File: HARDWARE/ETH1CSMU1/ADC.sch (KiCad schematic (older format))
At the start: 25 parts, among them U1201 AD746, U1202 LTC6655-5, U1203 LTC2512-24, U1204 OP07, U1205 ADG5204_TSSOP

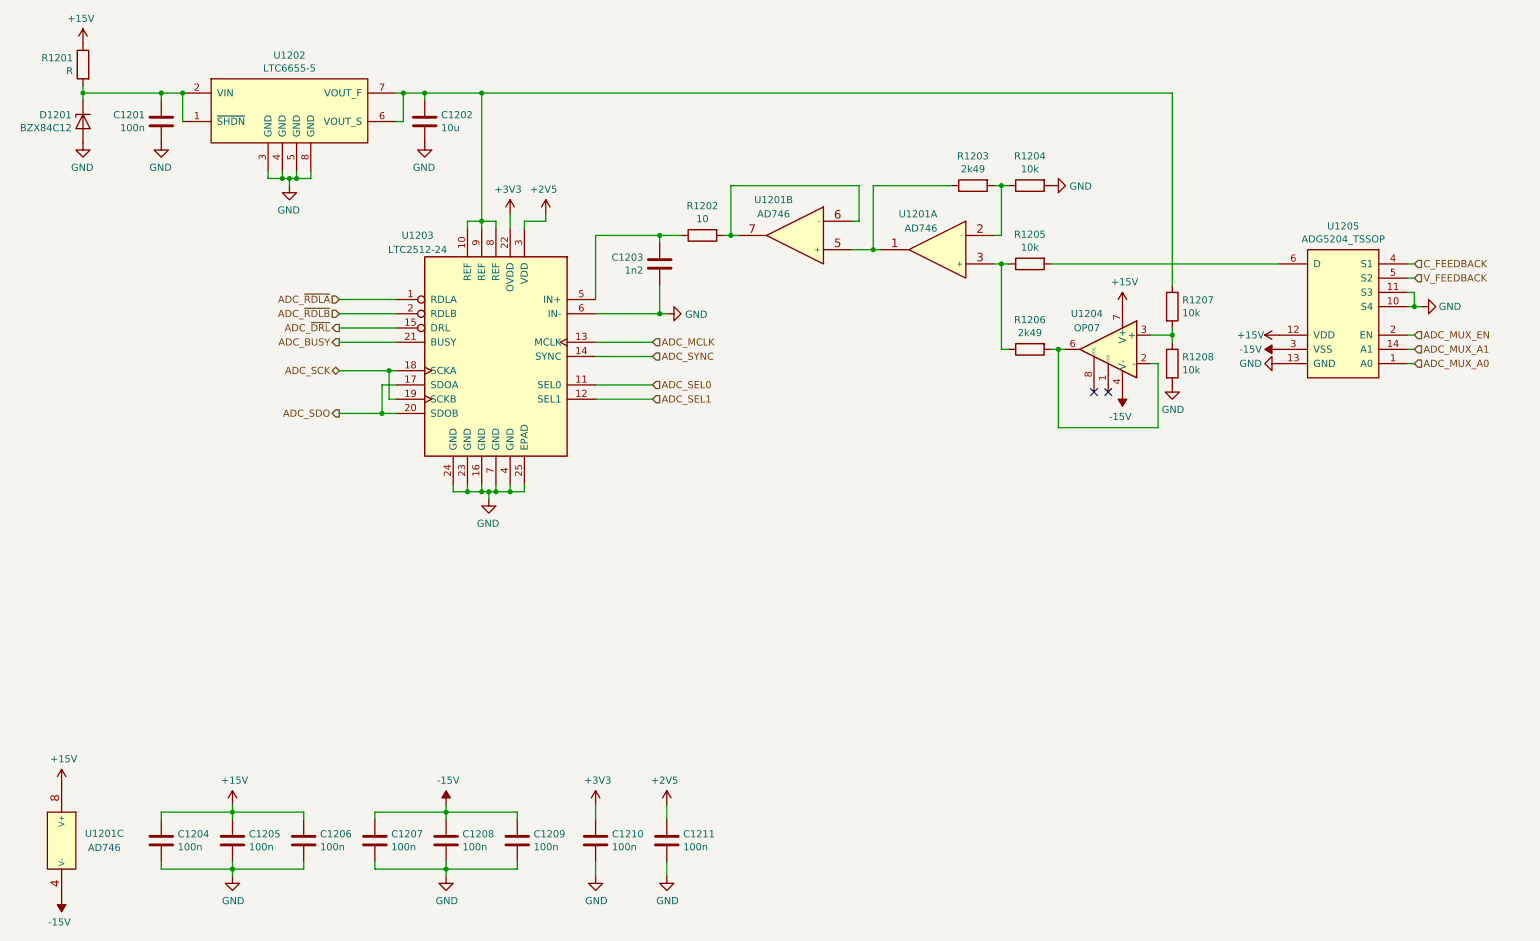
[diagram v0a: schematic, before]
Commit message: Commit
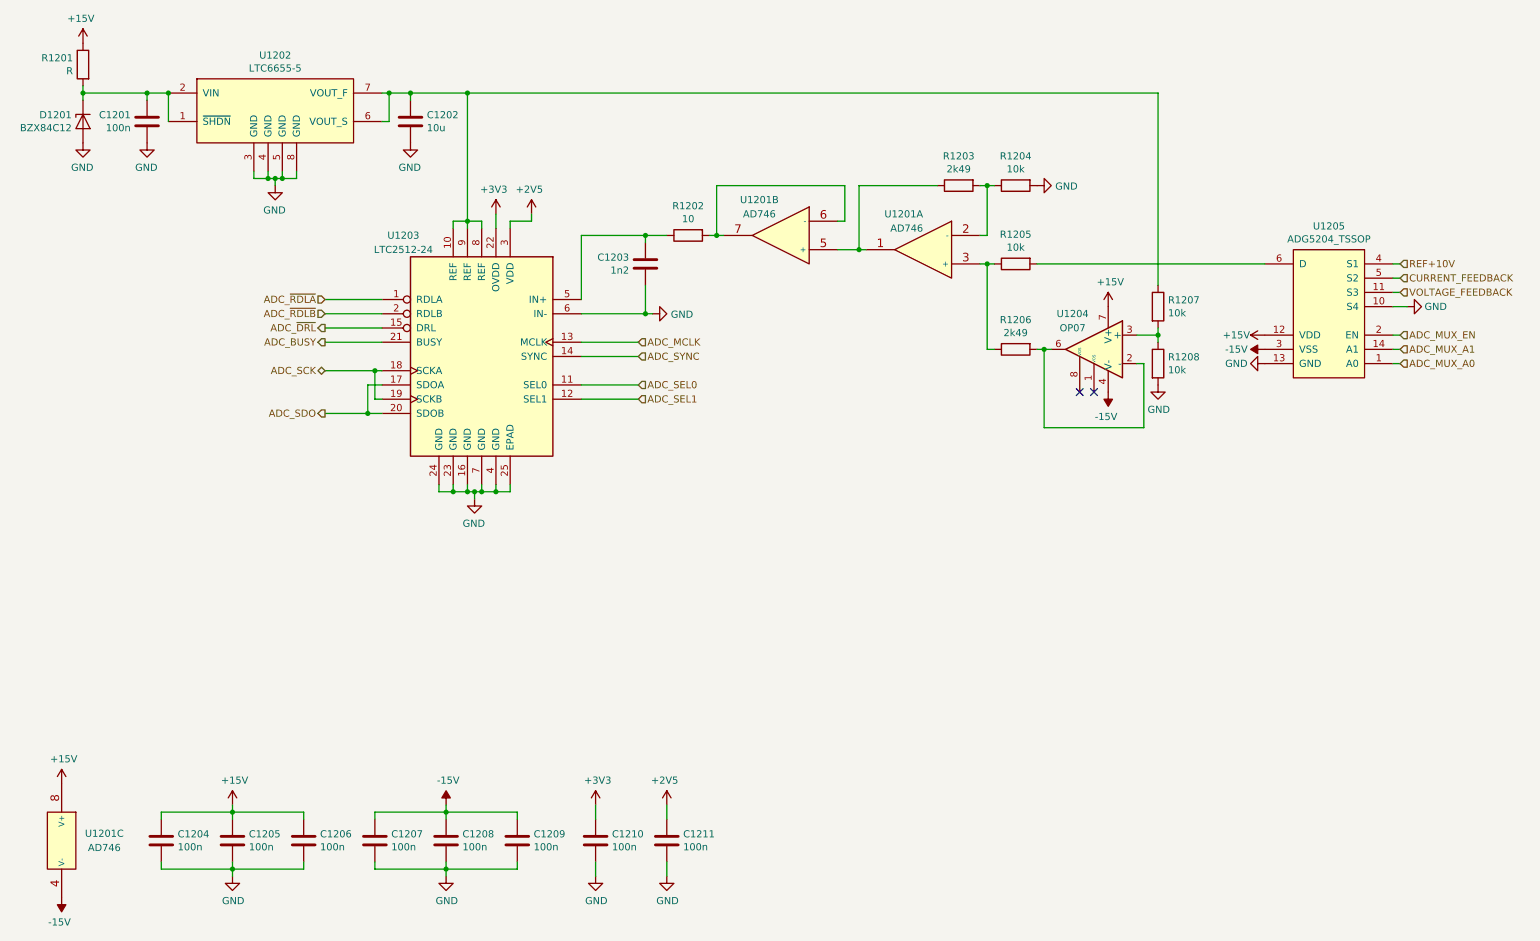
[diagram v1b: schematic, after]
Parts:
- C1201, C1204, C1205, C1206, C1207, C1208, C1209, C1210, C1211: footprint (none) -> SMD:C_0603_Symbol1
- R1204, R1205, R1207, R1208: footprint (none) -> SMD:R_0603_Symbol1
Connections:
- net GND: no longer U1205.11 (S3)
- net C_FEEDBACK renamed REF+10V
- net V_FEEDBACK renamed CURRENT_FEEDBACK
- new net VOLTAGE_FEEDBACK: U1205.11 (S3)
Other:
- moved on the sheet: C1201, C1202, C1203, R1202, R1203, R1204, R1205, R1206, R1207, R1208, U1201A, U1201B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

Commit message: Footprints
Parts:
- C1203: footprint (none) -> Capacitors_SMD:C_0603
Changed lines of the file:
@@
 F 0 "C1203" H 5115 2996 50  0000 L CNN
 F 1 "1n2" H 5115 2905 50  0000 L CNN
-F 2 "" H 5038 2800 50  0001 C CNN
+F 2 "Capacitors_SMD:C_0603" H 5038 2800 50  0001 C CNN
 F 3 "~" H 5000 2950 50  0001 C CNN
 	1    5000 2950

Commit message: Footprint selection
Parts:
- R1201, R1202, R1203, R1206: footprint (none) -> Resistors_SMD:R_0603
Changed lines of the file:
@@
 F 0 "R1202" V 5093 2750 50  0000 C CNN
 F 1 "10" V 5184 2750 50  0000 C CNN
-F 2 "" V 5230 2750 50  0001 C CNN
+F 2 "Resistors_SMD:R_0603" V 5230 2750 50  0001 C CNN
 F 3 "~" H 5300 2750 50  0001 C CNN
 	1    5300 2750
@@
 F 0 "R1201" H 1120 1596 50  0000 L CNN
 F 1 "R" H 1120 1505 50  0000 L CNN
-F 2 "" V 980 1550 50  0001 C CNN
+F 2 "Resistors_SMD:R_0603" V 980 1550 50  0001 C CNN
 F 3 "~" H 1050 1550 50  0001 C CNN
 	1    1050 1550
@@
 F 0 "R1203" V 6993 2400 50  0000 C CNN
 F 1 "2k49" V 7084 2400 50  0000 C CNN
-F 2 "" V 7130 2400 50  0001 C CNN
+F 2 "Resistors_SMD:R_0603" V 7130 2400 50  0001 C CNN
 F 3 "~" H 7200 2400 50  0001 C CNN
 	1    7200 2400
@@
 F 0 "R1206" V 7393 3550 50  0000 C CNN
 F 1 "2k49" V 7484 3550 50  0000 C CNN
-F 2 "" V 7530 3550 50  0001 C CNN
+F 2 "Resistors_SMD:R_0603" V 7530 3550 50  0001 C CNN
 F 3 "~" H 7600 3550 50  0001 C CNN
 	1    7600 3550
